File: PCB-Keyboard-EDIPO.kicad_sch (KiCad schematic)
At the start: 21 parts, among them J1 AVR-ISP-6, SW68 SW_Push_Reset, U1 ATmega32U4-A, U2 PRTR5V0U2X, Y1 XTAL

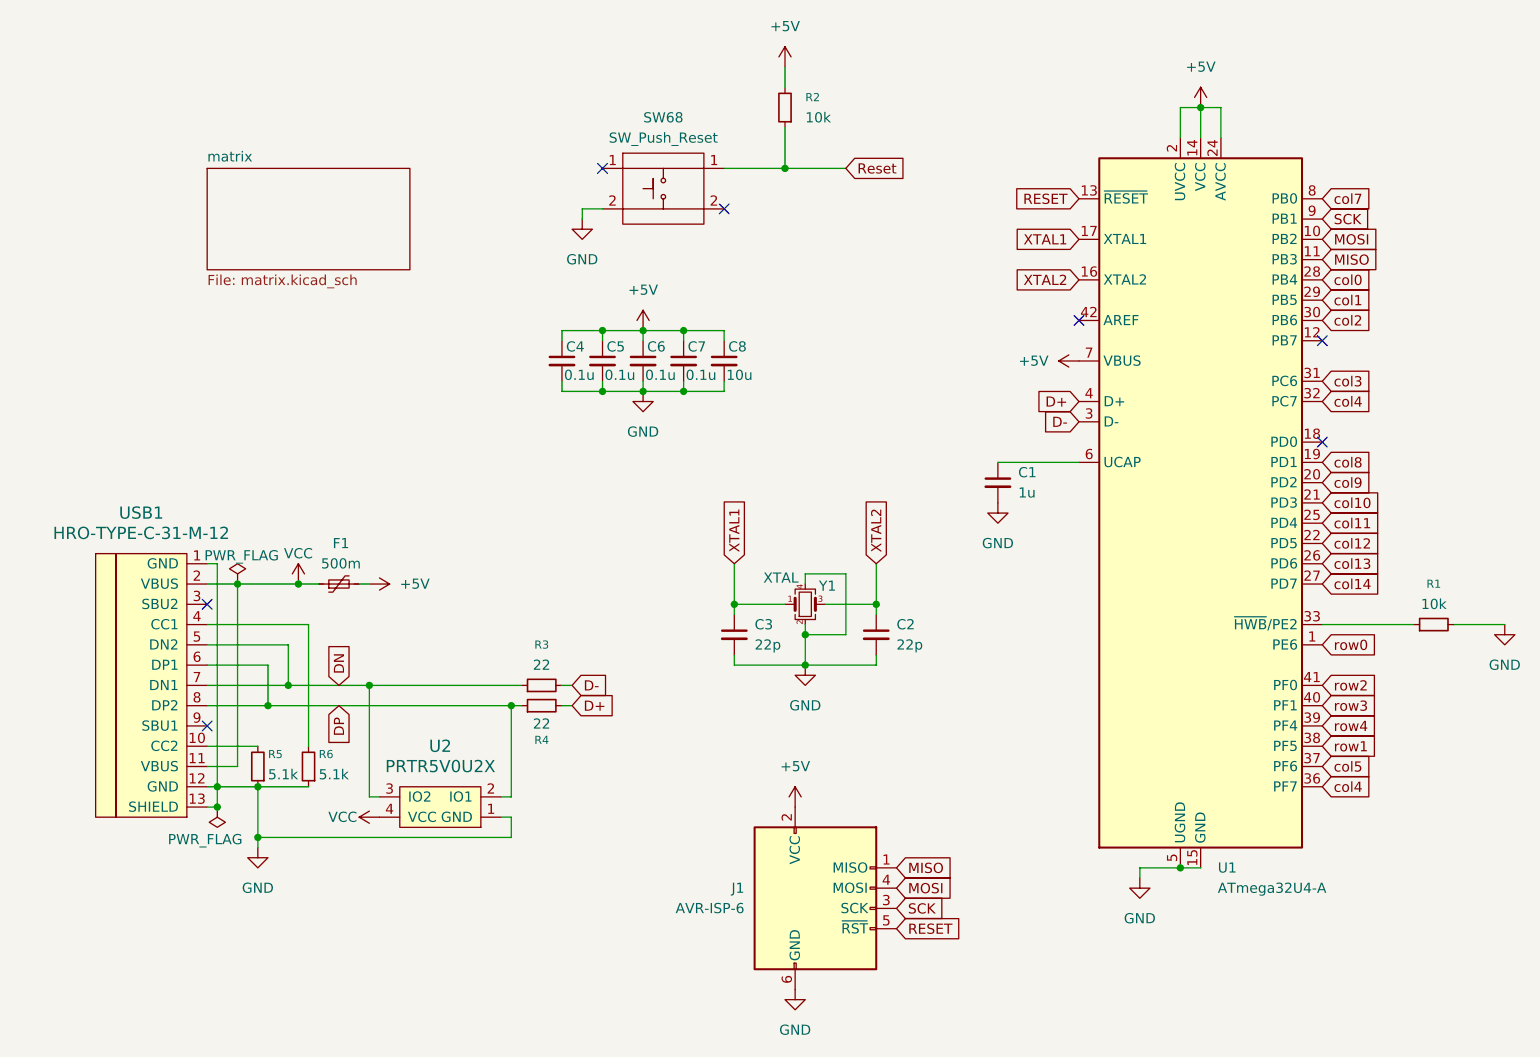
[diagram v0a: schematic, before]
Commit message: PCB Component Movement 1
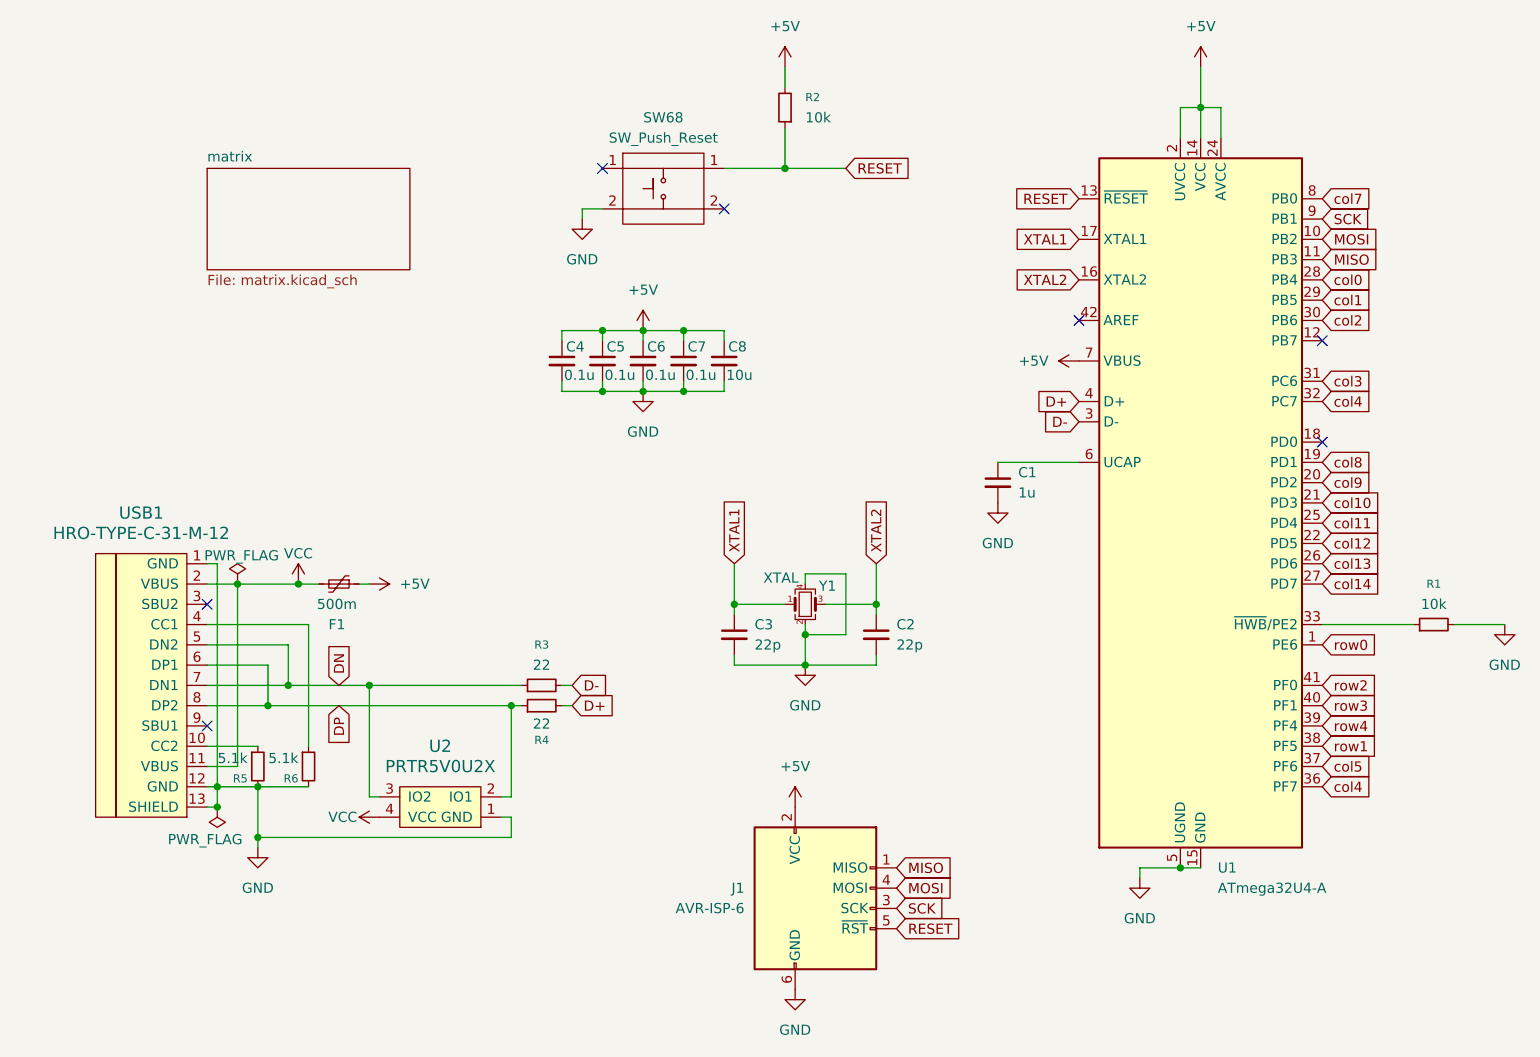
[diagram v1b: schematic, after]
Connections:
- net Reset is gone; now on net RESET: R2.1, SW68.1
- net +5V: now also F1.1; no longer F1.2
- net GND: now also R5.2, R6.2; no longer R5.1, R6.1
- net VCC: now also F1.2; no longer F1.1
- net at USB1.10 (CC2): now also R5.1; no longer R5.2
- net at USB1.4 (CC1): now also R6.1; no longer R6.2
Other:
- moved on the sheet: F1, R5, R6
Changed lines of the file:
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@@
 	)
 	(junction
+		(at 213.36 30.48)
+		(diameter 0)
+		(color 0 0 0 0)
+	)
+	(junction
 		(at 143.51 66.04)
 		(diameter 0)
@@
 		(color 0 0 0 0)
 	)
-	(junction
-		(at 213.36 30.48)
-		(diameter 0)
-		(color 0 0 0 0)
-	)
 	(no_connect
 		(at 88.9 92.71)
@@
 	(wire
 		(pts
+			(xy 215.9 34.29) (xy 215.9 30.48)
+		)
+		(stroke
+			(width 0)
+			(type default)
+		)
+	)
+	(wire
+		(pts
 			(xy 245.11 95.25) (xy 251.46 95.25)
 		)
@@
 	(wire
 		(pts
+			(xy 213.36 30.48) (xy 213.36 34.29)
+		)
+		(stroke
+			(width 0)
+			(type default)
+		)
+	)
+	(wire
+		(pts
 			(xy 96.52 100.33) (xy 96.52 105.41)
 		)
@@
 	(wire
 		(pts
+			(xy 213.36 25.4) (xy 213.36 30.48)
+		)
+		(stroke
+			(width 0)
+			(type default)
+		)
+	)
+	(wire
+		(pts
 			(xy 161.29 33.02) (xy 161.29 38.1)
 		)
@@
 	(wire
 		(pts
-			(xy 215.9 30.48) (xy 215.9 34.29)
+			(xy 133.35 105.41) (xy 134.62 105.41)
 		)
 		(stroke
@@
 	(wire
 		(pts
-			(xy 133.35 105.41) (xy 134.62 105.41)
+			(xy 138.43 58.42) (xy 138.43 59.69)
 		)
 		(stroke
@@
 	(wire
 		(pts
-			(xy 138.43 58.42) (xy 138.43 59.69)
+			(xy 95.25 115.57) (xy 95.25 121.92)
 		)
 		(stroke
@@
 	(wire
 		(pts
-			(xy 95.25 115.57) (xy 95.25 121.92)
+			(xy 210.82 34.29) (xy 210.82 30.48)
 		)
 		(stroke
@@
 	(wire
 		(pts
-			(xy 213.36 30.48) (xy 213.36 34.29)
-		)
-		(stroke
-			(width 0)
-			(type default)
-		)
-	)
-	(wire
-		(pts
 			(xy 163.83 96.52) (xy 163.83 100.33)
 		)
@@
 	(wire
 		(pts
-			(xy 210.82 30.48) (xy 213.36 30.48)
-		)
-		(stroke
-			(width 0)
-			(type default)
-		)
-	)
-	(wire
-		(pts
 			(xy 135.89 43.18) (xy 135.89 44.45)
 		)
@@
 	(wire
 		(pts
-			(xy 210.82 34.29) (xy 210.82 30.48)
+			(xy 88.9 102.87) (xy 99.06 102.87)
 		)
 		(stroke
@@
 	(wire
 		(pts
-			(xy 88.9 102.87) (xy 99.06 102.87)
+			(xy 133.35 64.77) (xy 133.35 66.04)
 		)
 		(stroke
@@
 	(wire
 		(pts
-			(xy 133.35 64.77) (xy 133.35 66.04)
+			(xy 172.72 100.33) (xy 172.72 99.06)
 		)
 		(stroke
@@
 	(wire
 		(pts
-			(xy 172.72 100.33) (xy 172.72 99.06)
+			(xy 148.59 58.42) (xy 153.67 58.42)
 		)
 		(stroke
@@
 	(wire
 		(pts
-			(xy 148.59 58.42) (xy 153.67 58.42)
+			(xy 168.91 96.52) (xy 168.91 88.9)
 		)
 		(stroke
@@
 	(wire
 		(pts
-			(xy 168.91 96.52) (xy 168.91 88.9)
+			(xy 138.43 64.77) (xy 138.43 66.04)
 		)
 		(stroke
@@
 	(wire
 		(pts
-			(xy 138.43 64.77) (xy 138.43 66.04)
+			(xy 210.82 30.48) (xy 213.36 30.48)
 		)
 		(stroke
@@
 	(wire
 		(pts
-			(xy 213.36 30.48) (xy 215.9 30.48)
+			(xy 154.94 99.06) (xy 154.94 100.33)
 		)
 		(stroke
@@
 	(wire
 		(pts
-			(xy 154.94 99.06) (xy 154.94 100.33)
+			(xy 215.9 30.48) (xy 213.36 30.48)
 		)
 		(stroke
@@
 		)
 	)
-	(global_label "Reset"
+	(global_label "RESET"
 		(shape input)
 		(at 168.91 38.1 0)
@@
 	(symbol
 		(lib_id "power:+5V")
-		(at 213.36 30.48 0)
+		(at 213.36 25.4 0)
 		(unit 1)
 		(exclude_from_sim no)
@@
 		(fields_autoplaced yes)
 		(property "Reference" "#PWR01"
-			(at 213.36 34.29 0)
+			(at 213.36 29.21 0)
 			(effects
 				(font
@@
 		)
 		(property "Value" "+5V"
-			(at 213.36 25.4 0)
+			(at 213.36 20.32 0)
 			(effects
 				(font
@@
 		)
 		(property "Footprint" ""
-			(at 213.36 30.48 0)
+			(at 213.36 25.4 0)
 			(effects
 				(font
@@
 		)
 		(property "Datasheet" ""
-			(at 213.36 30.48 0)
+			(at 213.36 25.4 0)
 			(effects
 				(font
@@
 		)
 		(property "Description" "Power symbol creates a global label with name \"+5V\""
-			(at 213.36 30.48 0)
+			(at 213.36 25.4 0)
 			(effects
 				(font
@@
 	(symbol
 		(lib_id "Device:Polyfuse_Small")
-		(at 105.41 90.17 90)
+		(at 105.41 90.17 270)
 		(unit 1)
 		(exclude_from_sim no)
@@
 		(dnp no)
 		(property "Reference" "F1"
-			(at 105.664 85.09 90)
+			(at 105.156 95.25 90)
 			(effects
 				(font
@@
 		)
 		(property "Value" "500m"
-			(at 105.664 87.63 90)
+			(at 105.156 92.71 90)
 			(effects
 				(font
@@
 		)
 		(property "Footprint" "Fuse:Fuse_1206_3216Metric_Pad1.42x1.75mm_HandSolder"
-			(at 110.49 88.9 0)
+			(at 100.33 91.44 0)
 			(effects
 				(font
@@
 	(symbol
 		(lib_id "Device:R_Small")
-		(at 95.25 113.03 180)
+		(at 95.25 113.03 0)
 		(unit 1)
 		(exclude_from_sim no)
@@
 		(dnp no)
 		(property "Reference" "R5"
-			(at 96.52 111.506 0)
+			(at 93.98 114.554 0)
 			(effects
 				(font
@@
 		)
 		(property "Value" "5.1k"
-			(at 96.52 114.046 0)
+			(at 93.98 112.014 0)
 			(effects
 				(font
@@
 	(symbol
 		(lib_id "Device:R_Small")
-		(at 101.6 113.03 180)
+		(at 101.6 113.03 0)
 		(unit 1)
 		(exclude_from_sim no)
@@
 		(dnp no)
 		(property "Reference" "R6"
-			(at 102.87 111.506 0)
+			(at 100.33 114.554 0)
 			(effects
 				(font
@@
 		)
 		(property "Value" "5.1k"
-			(at 102.87 114.046 0)
+			(at 100.33 112.014 0)
 			(effects
 				(font
